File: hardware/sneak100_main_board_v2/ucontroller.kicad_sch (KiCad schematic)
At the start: 27 parts, among them J1 USB_B_Mini, J2 Conn_02x05_Odd_Even, J3 Conn_01x03, SW1 SW_DIP_x04, SW2 SW_Push, U1 STM32F405RGTx, Y1 8MHz

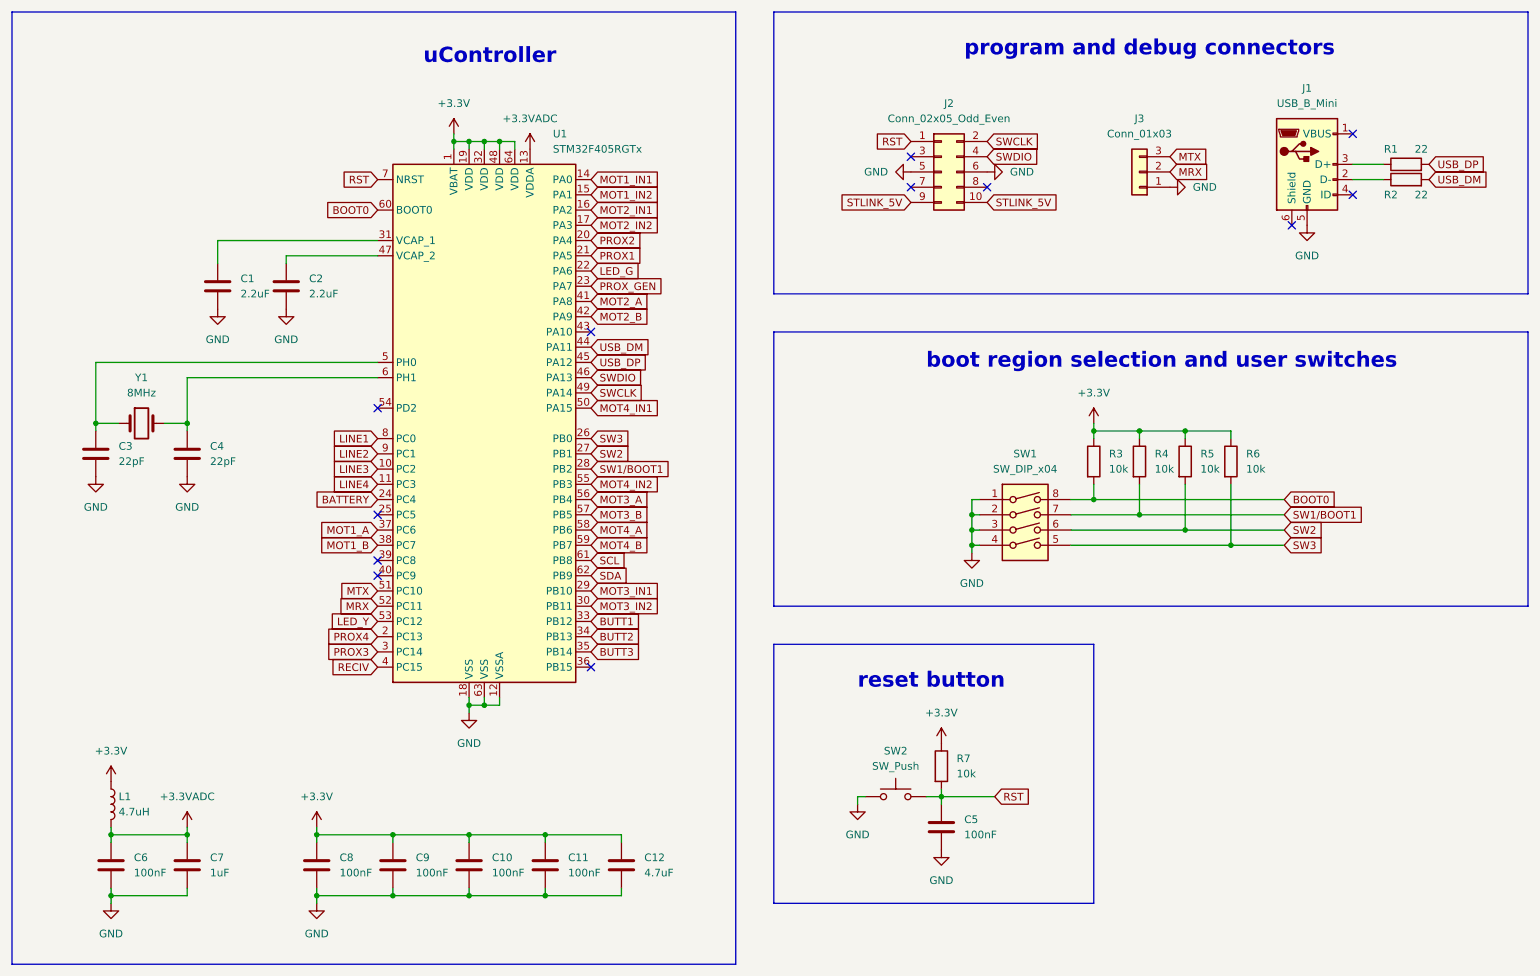
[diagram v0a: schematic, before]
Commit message: small improvements
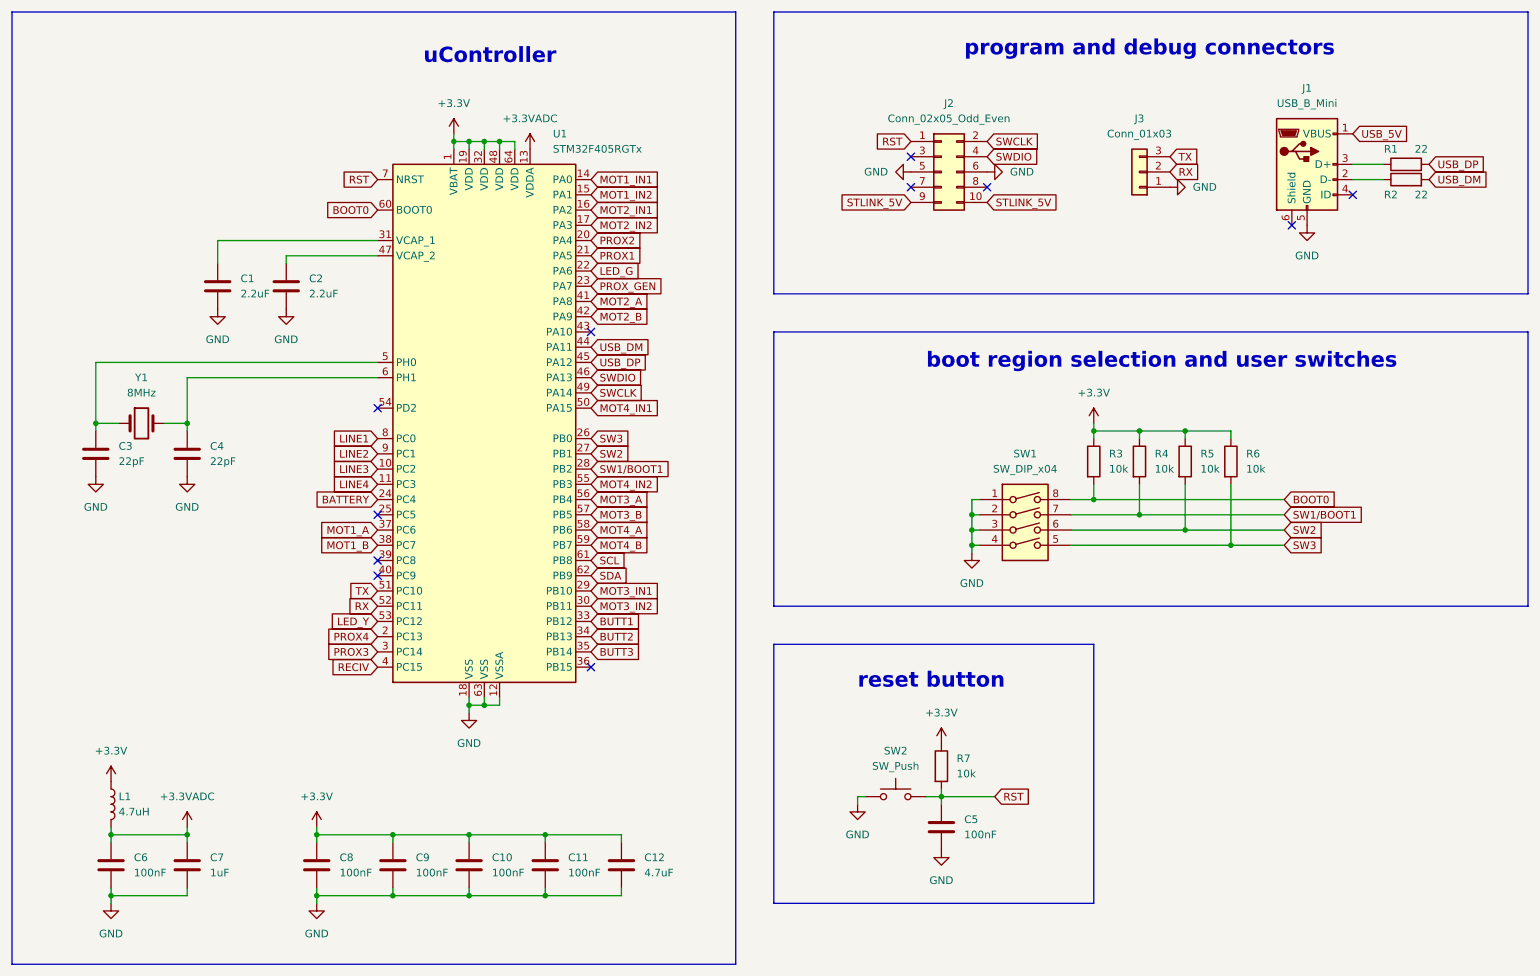
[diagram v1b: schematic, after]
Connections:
- net USB_5V: now reaches J1.1 (VBUS)
- net MRX renamed RX
- net MTX renamed TX
- no-connect marks 12 -> 11
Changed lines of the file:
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@@
   (no_connect (at 119.38 124.46))
   (no_connect (at 246.38 45.72))
-  (no_connect (at 246.38 35.56))
   (no_connect (at 83.82 109.22))
   (no_connect (at 83.82 106.68))
@@
     )
   )
-  (global_label "MTX" (shape input) (at 83.82 111.76 180) (fields_autoplaced)
-    (effects (font (size 1.27 1.27)) (justify right))
-    (property "Intersheet References" "${INTERSHEET_REFS}" (id 0) (at 77.7783 111.6806 0)
+  (global_label "TX" (shape input) (at 83.82 111.76 180) (fields_autoplaced)
+    (effects (font (size 1.27 1.27)) (justify right))
+    (property "Intersheet References" "${INTERSHEET_REFS}" (id 0) (at 79.2298 111.6806 0)
       (effects (font (size 1.27 1.27)) (justify right) hide)
     )
@@
     )
   )
-  (global_label "MRX" (shape input) (at 83.82 114.3 180) (fields_autoplaced)
-    (effects (font (size 1.27 1.27)) (justify right))
-    (property "Intersheet References" "${INTERSHEET_REFS}" (id 0) (at 77.4759 114.2206 0)
+  (global_label "RX" (shape input) (at 83.82 114.3 180) (fields_autoplaced)
+    (effects (font (size 1.27 1.27)) (justify right))
+    (property "Intersheet References" "${INTERSHEET_REFS}" (id 0) (at 78.9274 114.2206 0)
       (effects (font (size 1.27 1.27)) (justify right) hide)
     )
@@
     )
   )
-  (global_label "MRX" (shape input) (at 215.9 41.91 0) (fields_autoplaced)
-    (effects (font (size 1.27 1.27)) (justify left))
-    (property "Intersheet References" "${INTERSHEET_REFS}" (id 0) (at 222.2441 41.9894 0)
+  (global_label "RX" (shape input) (at 215.9 41.91 0) (fields_autoplaced)
+    (effects (font (size 1.27 1.27)) (justify left))
+    (property "Intersheet References" "${INTERSHEET_REFS}" (id 0) (at 220.7926 41.8306 0)
       (effects (font (size 1.27 1.27)) (justify left) hide)
     )
@@
     )
   )
-  (global_label "MTX" (shape input) (at 215.9 39.37 0) (fields_autoplaced)
-    (effects (font (size 1.27 1.27)) (justify left))
-    (property "Intersheet References" "${INTERSHEET_REFS}" (id 0) (at 221.9417 39.4494 0)
+  (global_label "TX" (shape input) (at 215.9 39.37 0) (fields_autoplaced)
+    (effects (font (size 1.27 1.27)) (justify left))
+    (property "Intersheet References" "${INTERSHEET_REFS}" (id 0) (at 220.4902 39.2906 0)
       (effects (font (size 1.27 1.27)) (justify left) hide)
     )
@@
       (effects (font (size 1.27 1.27)) (justify left) hide)
     )
+  )
+  (global_label "USB_5V" (shape input) (at 246.38 35.56 0) (fields_autoplaced)
+    (effects (font (size 1.27 1.27)) (justify left))
+    (property "Intersheet References" "${INTERSHEET_REFS}" (id 0) (at 255.8688 35.4806 0)
+      (effects (font (size 1.27 1.27)) (justify left) hide)
+    )
